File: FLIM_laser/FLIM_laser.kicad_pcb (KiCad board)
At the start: 2 copper layers, 28.6 x 25 mm, 22 parts, among them J1 Conn_01x02_Male, J2 Conn_01x02_Male, J3 Conn_01x02_Male, M1 EP2014C, U1 AMS1117-5.0, U2 LMG1020, U3 74LVC1G08

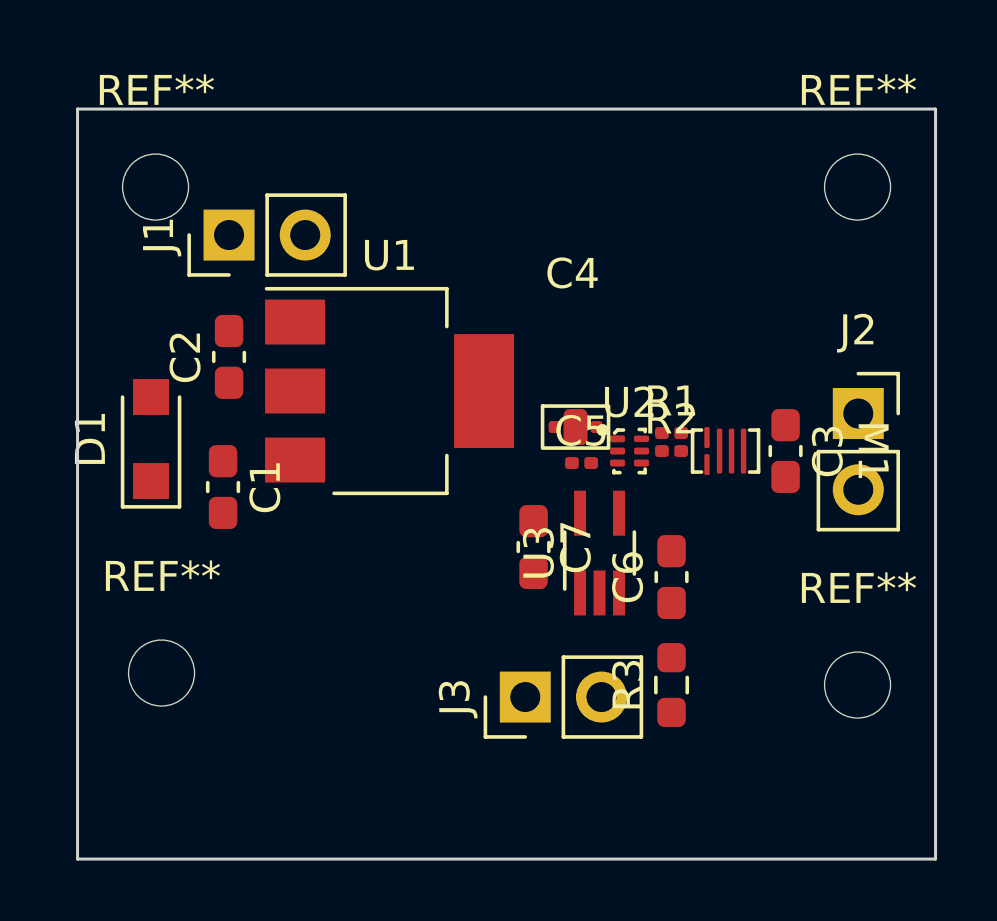
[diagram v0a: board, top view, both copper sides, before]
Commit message: v0.92 subcompleted
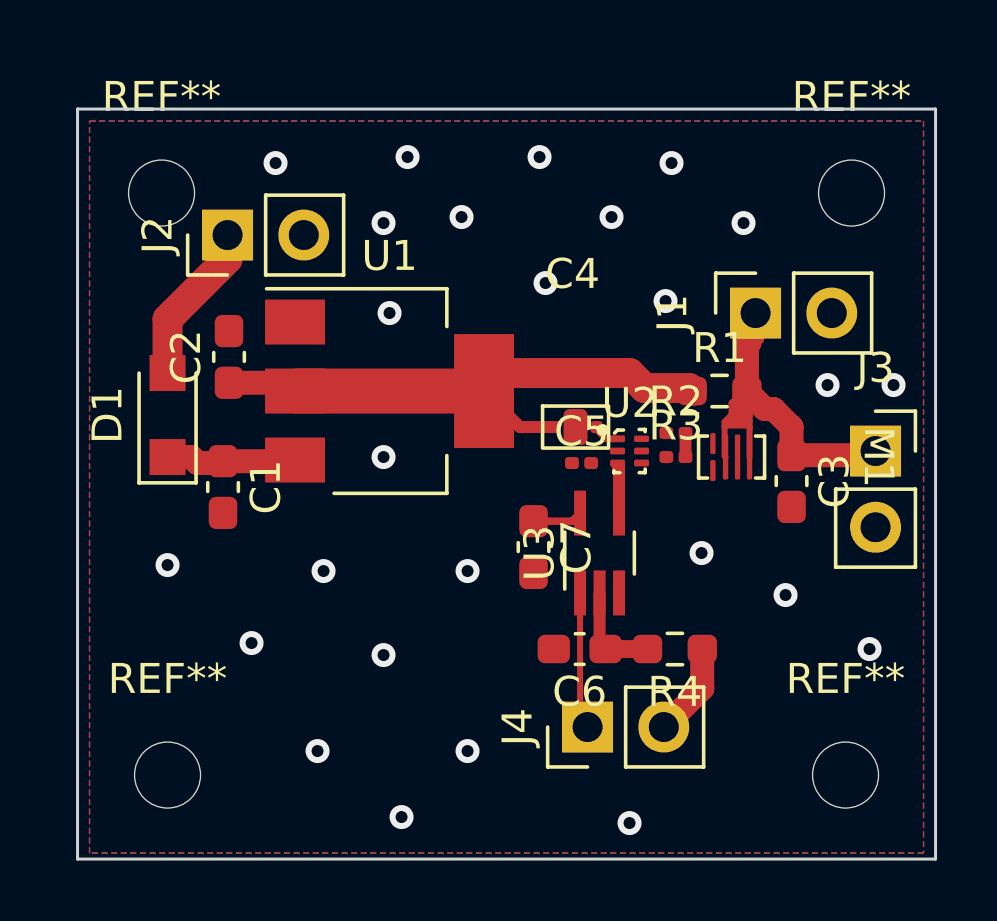
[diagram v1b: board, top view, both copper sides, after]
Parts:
- added J4: Conn_01x02_Male, Connector_PinHeader_2.54mm:PinHeader_1x02_P2.54mm_Vertical, F.Cu at (162.6, 59.2)
- added R4: R, Resistor_SMD:R_0603_1608Metric_Pad0.98x0.95mm_HandSolder, F.Cu at (165.5, 56.6)
- J1, J3: footprint Connector_PinHeader_2.54mm:PinHeader_1x02_P2.54mm_Vertical -> Connector_PinSocket_2.54mm:PinSocket_1x02_P2.54mm_Vertical
- J2: footprint Connector_PinSocket_2.54mm:PinSocket_1x02_P2.54mm_Vertical -> Connector_PinHeader_2.54mm:PinHeader_1x02_P2.54mm_Vertical
- R1: footprint Resistor_SMD:R_0201_0603Metric -> Resistor_SMD:R_0603_1608Metric_Pad0.98x0.95mm_HandSolder
- R3: footprint Resistor_SMD:R_0603_1608Metric_Pad0.98x0.95mm_HandSolder -> Resistor_SMD:R_0201_0603Metric
- moved J2 21.9 mm to (150.6, 42.8), turned to 90 degrees
- moved J1 17.7 mm to (168.2, 45.4)
- moved J3 14.3 mm to (172.2, 50.0), turned to 0 degrees
- moved R3 7.60 mm to (165.5, 50.2), turned to 0 degrees
- moved C6 3.89 mm to (162.3, 56.6), turned to 180 degrees
- moved REF** 3.41 mm to (148.6, 60.8)
- moved REF** 3.03 mm to (171.2, 60.8)
- moved R1 2.13 mm to (167.0, 48.0)
- moved C3 1.02 mm to (169.4, 51.0)
- moved D1 0.97 mm to (148.6, 48.8)
- moved R2 0.62 mm to (165.5, 49.4)
- moved M1 0.28 mm to (166.8, 50.2)
- moved REF** 0.28 mm to (148.4, 41.4)
- moved REF** 0.28 mm to (171.4, 41.4)
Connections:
- C3 pad 1: +5V -> Net-(C3-Pad1)
- J1 pad 1: Net-(D1-Pad2) -> Net-(C3-Pad1)
- J2 pad 1: +5V -> Net-(D1-Pad2)
- J3 pad 1: Net-(J3-Pad1) -> Net-(C3-Pad1)
- J3 pad 2: Net-(J3-Pad2) -> GND
- M1 pad 3: +5V -> Net-(C3-Pad1)
- M1 pad 5: +5V -> Net-(C3-Pad1)
- R1 pad 1: Net-(R1-Pad1) -> +5V
- R1 pad 2: Net-(M1-Pad1) -> Net-(C3-Pad1)
- R3 pad 1: Net-(J3-Pad2) -> Net-(R3-Pad1)
- R3 pad 2: Net-(C6-Pad1) -> Net-(M1-Pad1)
- U2 pad A2: Net-(R1-Pad1) -> Net-(R2-Pad1)
- U2 pad B2: Net-(R2-Pad1) -> Net-(R3-Pad1)
- U3 pad 1: Net-(J3-Pad1) -> Net-(J4-Pad1)
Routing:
- net +5V: track 0.00 -> 22.3 mm
- net Net-(C3-Pad1): track 0.00 -> 18.8 mm
- net Net-(D1-Pad2): track 0.00 -> 5.43 mm
- net Net-(J4-Pad1): track 0.00 -> 4.59 mm
- net Net-(C1-Pad1): track 0.00 -> 4.57 mm
- net Net-(C6-Pad1): track 0.00 -> 3.35 mm
- net Net-(J4-Pad2): track 0.00 -> 3.13 mm
- net Net-(U2-PadC1): track 0.00 -> 1.58 mm
- net Net-(C4-Pad3): track 0.00 -> 0.87 mm
- net Net-(M1-Pad1): track 0.00 -> 0.80 mm
- net GND: vias 0 -> 26
- added copper zone on B.Cu, net GND
- added copper zone on F.Cu, net GND
